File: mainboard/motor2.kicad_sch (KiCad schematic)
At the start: 12 parts, among them U2 DRV8323RSRGZT

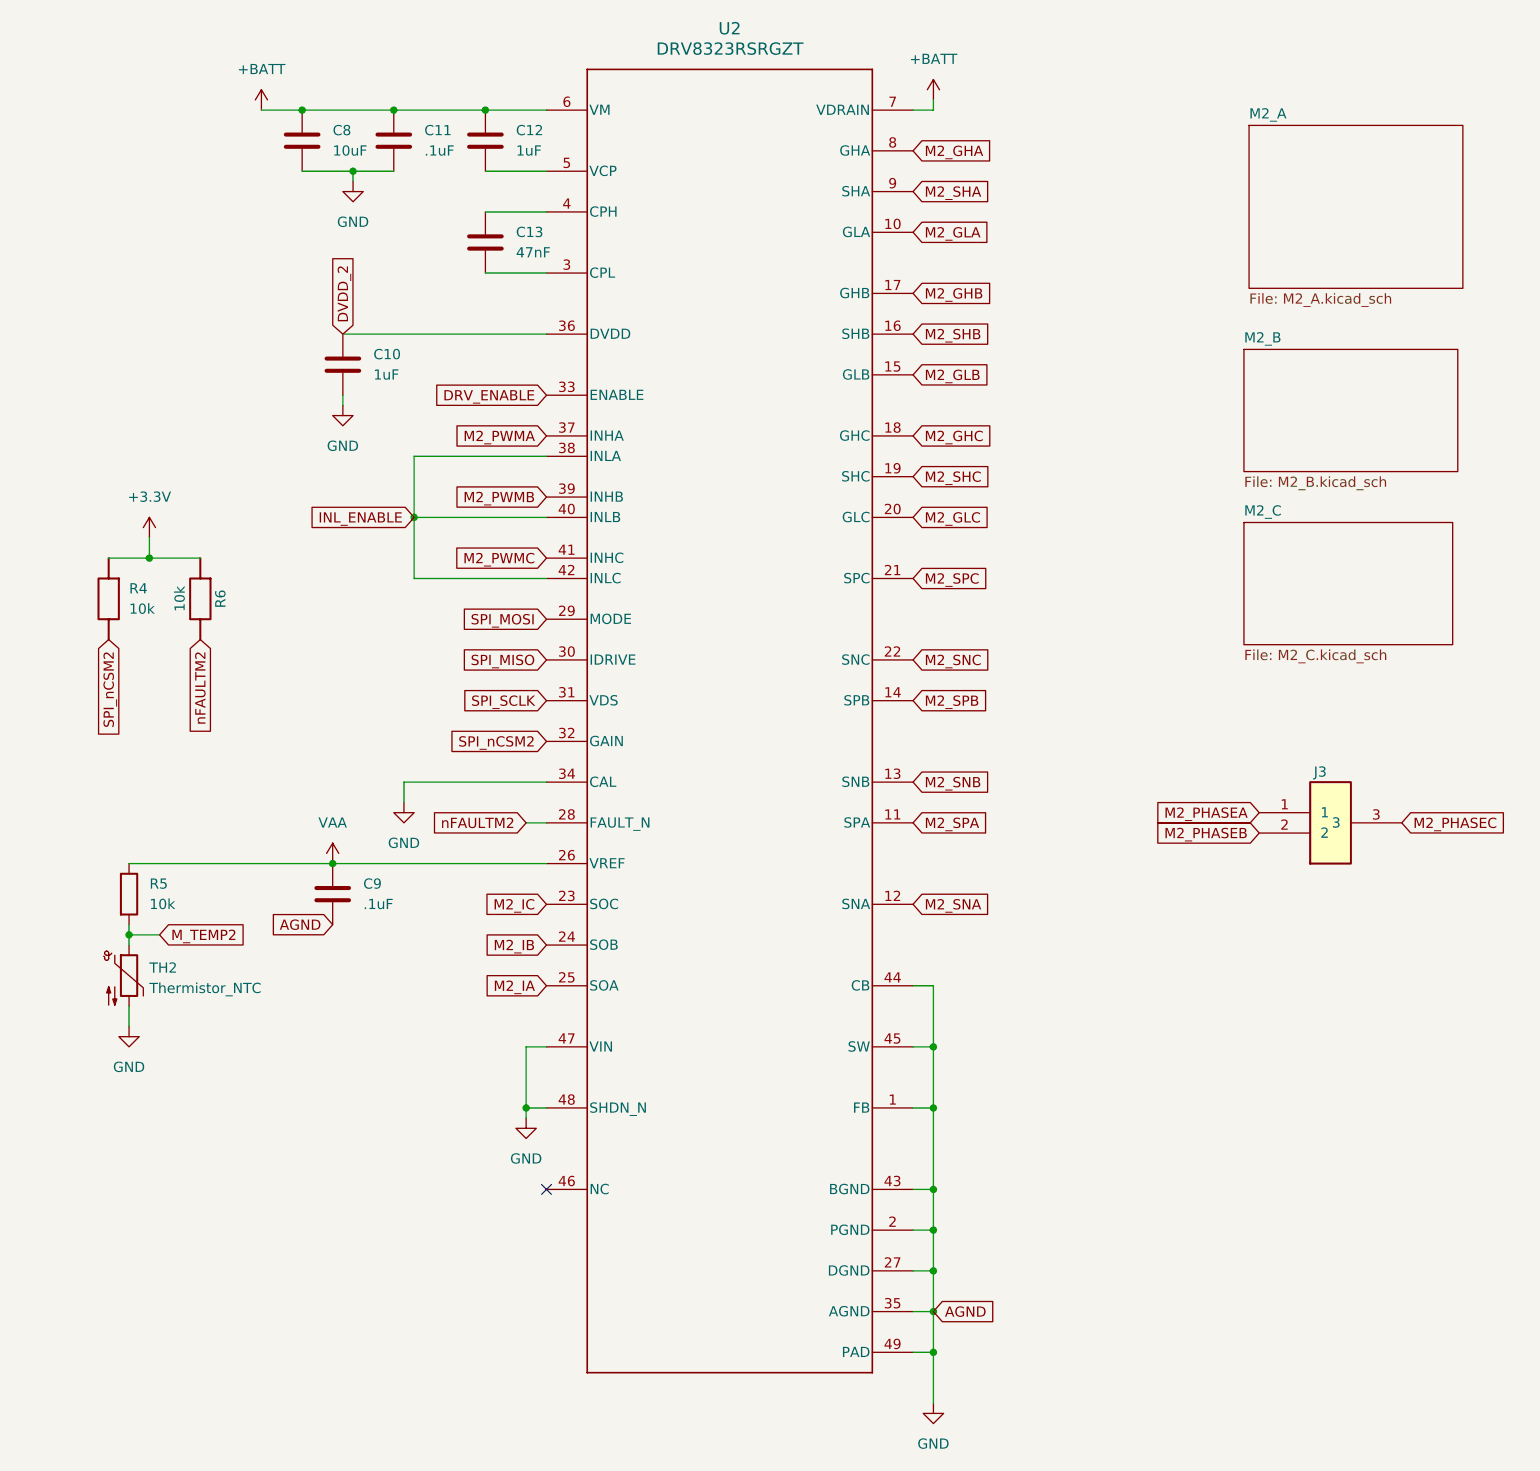
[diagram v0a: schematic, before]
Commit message: Initial layout completed
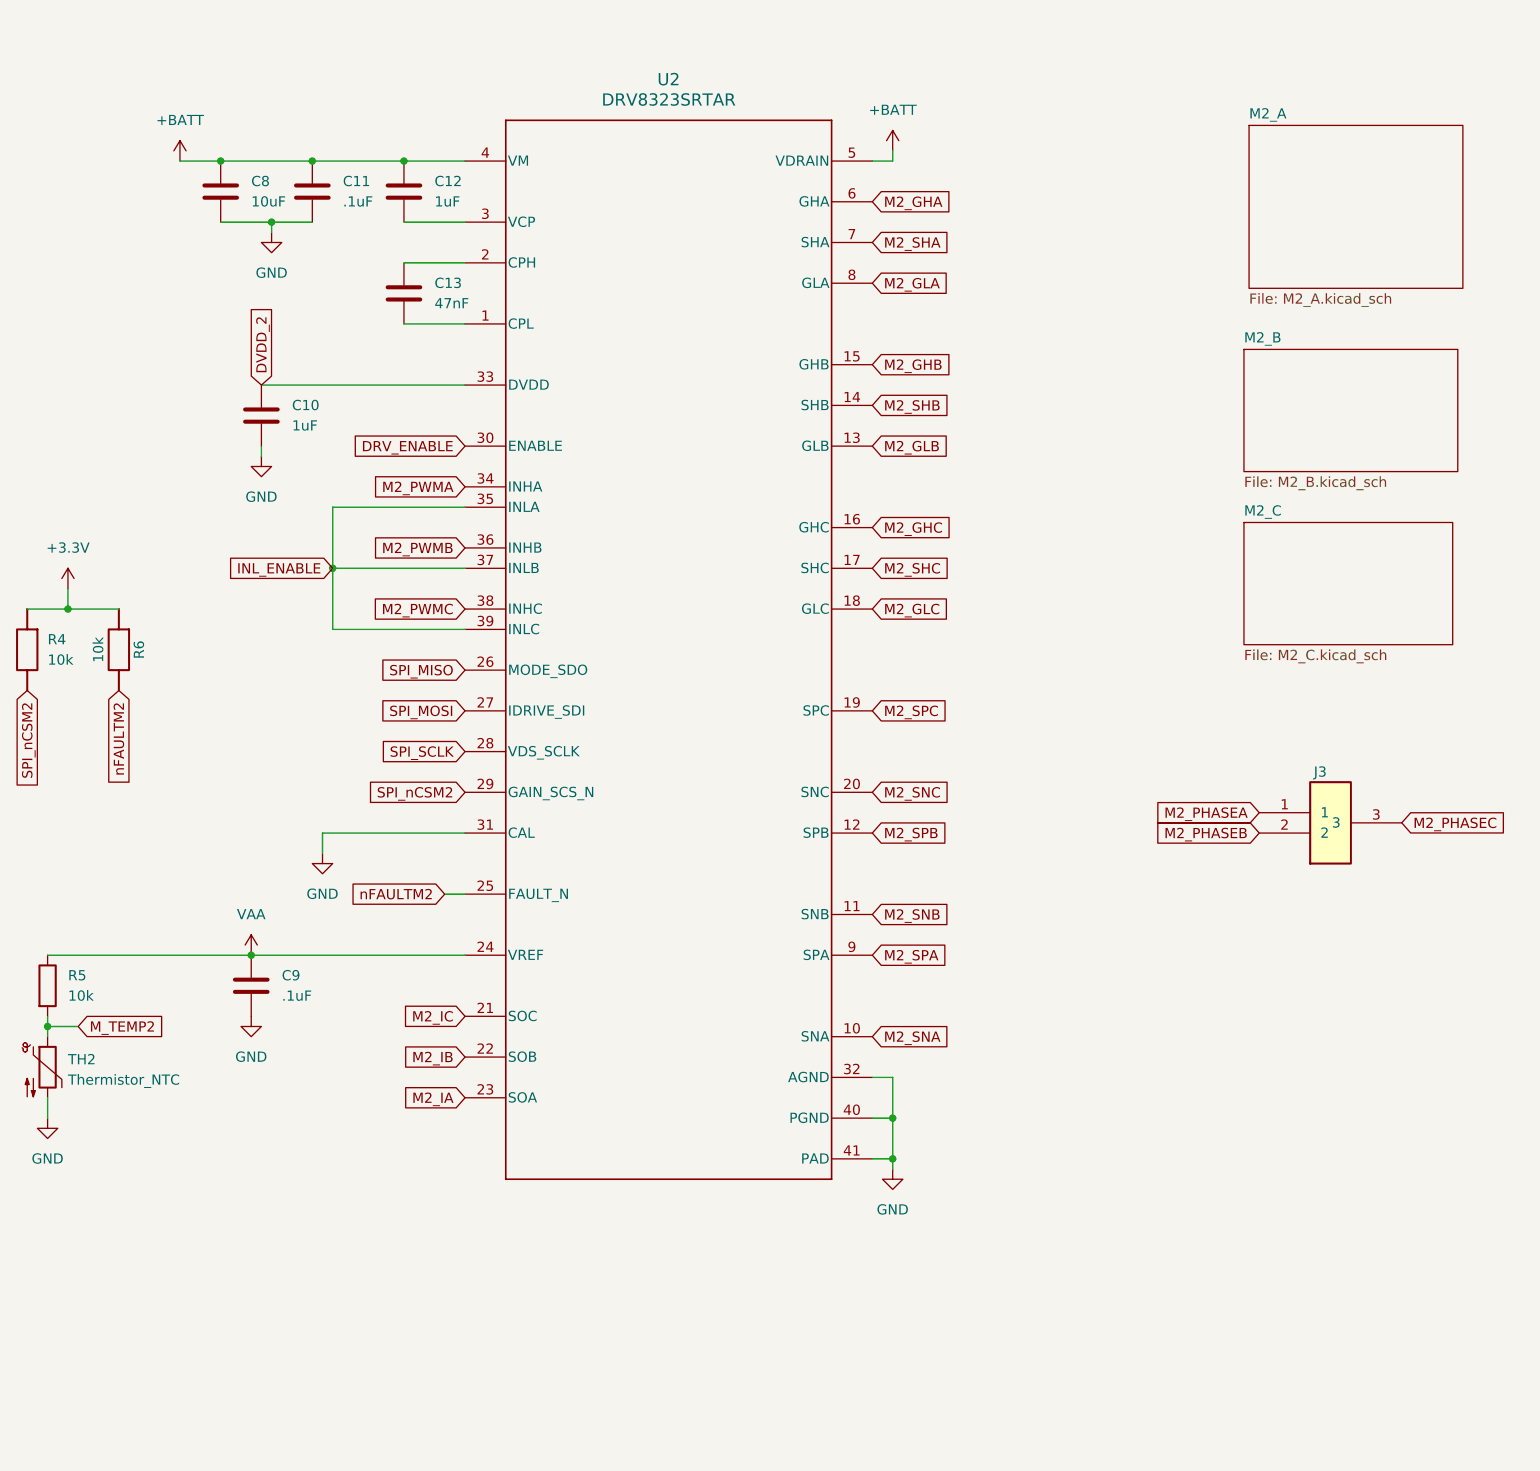
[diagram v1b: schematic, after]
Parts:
- removed U2: DRV8323RSRGZT, DRV8323RSRGZT_new:RGZ0048A, symbol DRV8323RSRGZT_new:DRV8323RSRGZT
- added U2: DRV8323SRTAR, DRV8323SRTAR:RTA0040B_NV, symbol DRV8323SR:DRV8323SRTAR
- C8: footprint Capacitor_SMD:C_1210_3225Metric -> Capacitor_SMD:C_1206_3216Metric
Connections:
- net +BATT: now also U2.4 (VM), U2.5 (VDRAIN)
- net DRV_ENABLE: now also U2.30 (ENABLE)
- net DVDD_2: now also U2.33 (DVDD)
- net GND: now also U2.31 (CAL), U2.32 (AGND), U2.40 (PGND), U2.41 (PAD)
- net INL_ENABLE: now also U2.35 (INLA), U2.37 (INLB), U2.39 (INLC)
- net M2_GHA: now also U2.6 (GHA)
- net M2_GHB: now also U2.15 (GHB)
- net M2_GHC: now also U2.16 (GHC)
- net M2_GLA: now also U2.8 (GLA)
- net M2_GLB: now also U2.13 (GLB)
- net M2_GLC: now also U2.18 (GLC)
- net M2_IA: now also U2.23 (SOA)
- net M2_IB: now also U2.22 (SOB)
- net M2_IC: now also U2.21 (SOC)
- net M2_PWMA: now also U2.34 (INHA)
- net M2_PWMB: now also U2.36 (INHB)
- net M2_PWMC: now also U2.38 (INHC)
- net M2_SHA: now also U2.7 (SHA)
- net M2_SHB: now also U2.14 (SHB)
- net M2_SHC: now also U2.17 (SHC)
- net M2_SNA: now also U2.10 (SNA)
- net M2_SNB: now also U2.11 (SNB)
- net M2_SNC: now also U2.20 (SNC)
- net M2_SPA: now also U2.9 (SPA)
- net M2_SPB: now also U2.12 (SPB)
- net M2_SPC: now also U2.19 (SPC)
- net SPI_MISO: now also U2.26 (MODE_SDO)
- net SPI_MOSI: now also U2.27 (IDRIVE_SDI)
- net SPI_SCLK: now also U2.28 (VDS_SCLK)
- net SPI_nCSM2: now also U2.29 (GAIN_SCS_N)
- net VAA: now also U2.24 (VREF)
- net nFAULTM2: now also U2.25 (FAULT_N)
- net at C12.2: now also U2.3 (VCP)
- net at C13.1: now also U2.2 (CPH)
- net at C13.2: now also U2.1 (CPL)
- no-connect marks 1 -> 0
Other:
- moved on the sheet: C10, C11, C12, C13, C8, C9, R4, R5, R6, TH2

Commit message: Use BeagleConnect product names consistently
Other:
- title: AM13E QuadESC Mainboard — Motor 2 -> BeagleConnect QuadESC Mainboard — Motor 2
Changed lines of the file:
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@@
 	(paper "USLetter")
 	(title_block
-		(title "AM13E QuadESC Mainboard — Motor 2")
+		(title "BeagleConnect QuadESC Mainboard — Motor 2")
 		(date "2026-08-06")
 		(rev "A")
